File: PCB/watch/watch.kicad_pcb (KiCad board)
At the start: 2 copper layers, 1 part

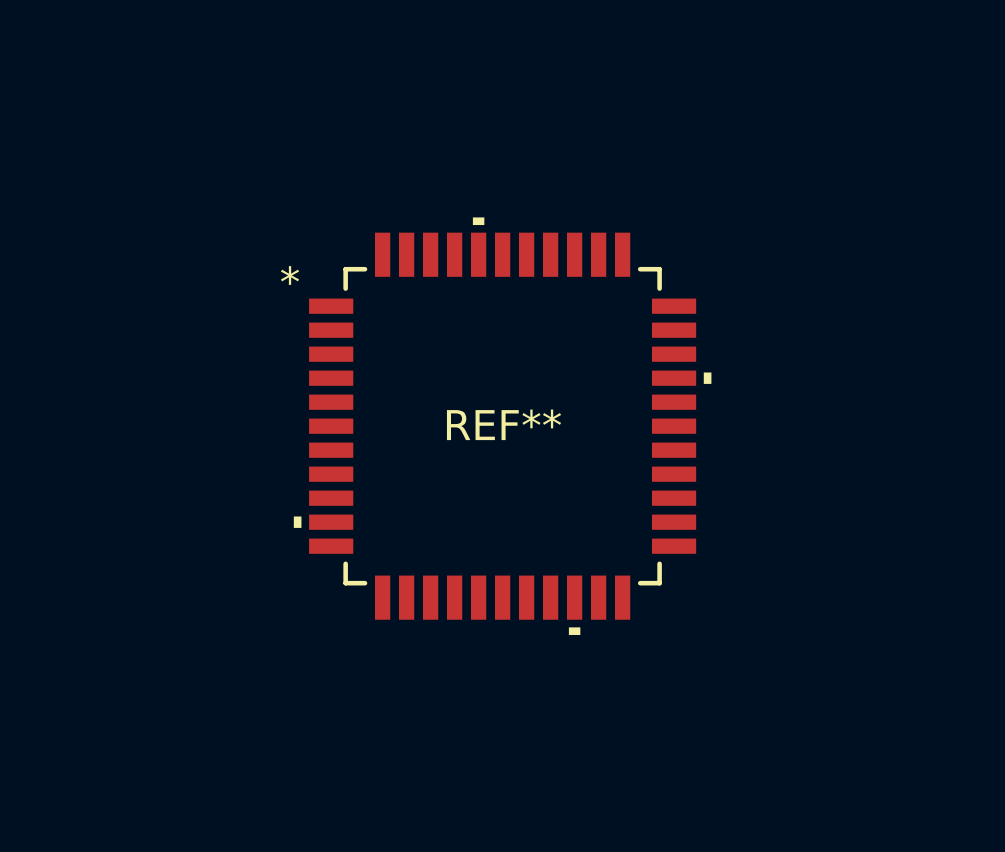
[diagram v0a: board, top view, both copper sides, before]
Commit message: feat(pcb): Buncha stuff happened
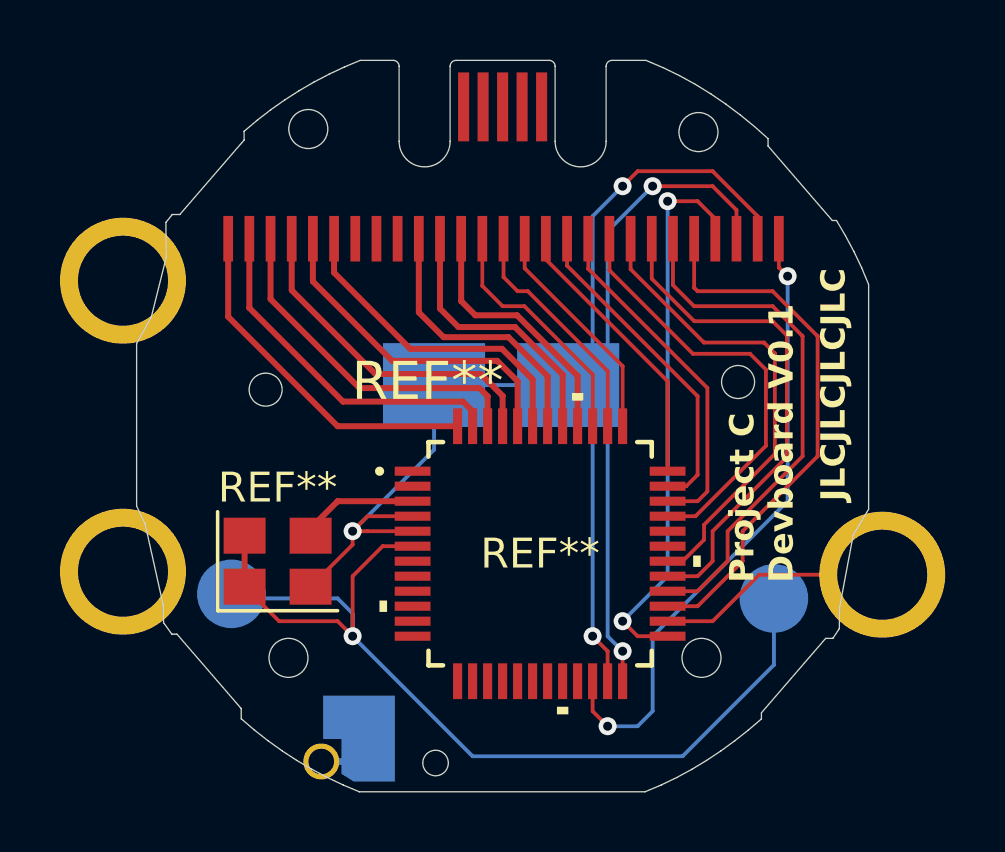
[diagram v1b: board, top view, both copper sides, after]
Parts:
- removed the REF** at (150.0, 100.0)
- added REF**: Val**, Casio Footprints:CASIO-F91W-OUTLINE, F.Cu at (150.0, 100.0)
- added REF**: Crystal_SMD_3225-4Pin_3.2x2.5mm, Crystal:Crystal_SMD_3225-4Pin_3.2x2.5mm, F.Cu at (142.5, 104.5)
- added REF**: LQFP48-7X7mm, STM8S105C6T6:LQFP48-7X7mm, F.Cu at (151.2, 104.2)
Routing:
- net (no net): track 0.00 -> 381.4 mm, vias 0 -> 10
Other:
- board outline added: 24.4 x 24.4 mm
- copper layers 2 -> 4
- board text added: "JLCJLCJLCJLC"
- board text added: "Project C Devboard V0.1"
